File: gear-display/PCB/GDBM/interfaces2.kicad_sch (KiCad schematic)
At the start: 1 part

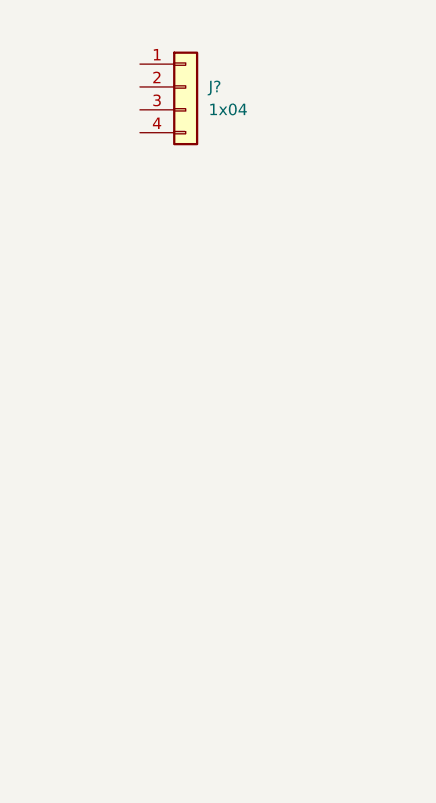
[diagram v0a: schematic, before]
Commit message: updates
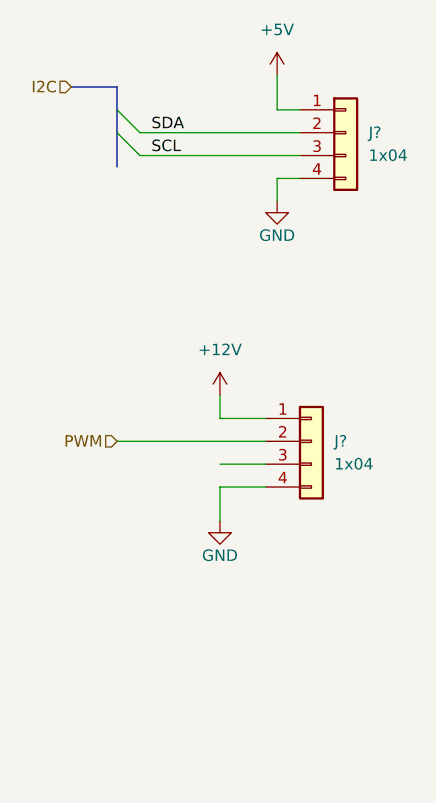
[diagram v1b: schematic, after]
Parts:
- added J?: Con_Screw_1x04_691313510004, KD_Connector_Screw:CON_508_1X04_691313510004_Mated, symbol KD_Connector_Screw:Con_Screw_1x04_691313510004
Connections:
- net +5V: now reaches J?.1 (Pin_1)
- net SDA: now reaches J?.2 (Pin_2)
- net SCL: now reaches J?.3 (Pin_3)
- net GND: now reaches J?.4 (Pin_4)
- net GND: now also J?.4 (Pin_4)
- new net +12V: J?.1 (Pin_1)
- new net PWM: J?.2 (Pin_2)
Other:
- moved on the sheet: J?
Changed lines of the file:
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@@
 (kicad_sch (version 20211123) (generator eeschema)
   (paper "A4")
-  (symbol (lib_id "KD_Connector_Screw:Con_Screw_1x04_691313510004") (at 166.37 53.34 0) (unit 1)
+  (bus_entry (at 163.83 58.42) (size 2.54 2.54)
+    (stroke (width 0) (type default) (color 0 0 0 0))
+  )
+  (bus_entry (at 163.83 60.96) (size 2.54 2.54)
+    (stroke (width 0) (type default) (color 0 0 0 0))
+  )
+  (wire (pts (xy 184.15 58.42) (xy 181.61 58.42))
+    (stroke (width 0) (type default) (color 0 0 0 0))
+  )
+  (bus (pts (xy 163.83 58.42) (xy 163.83 60.96))
+    (stroke (width 0) (type default) (color 0 0 0 0))
+  )
+  (wire (pts (xy 181.61 54.61) (xy 181.61 58.42))
+    (stroke (width 0) (type default) (color 0 0 0 0))
+  )
+  (wire (pts (xy 175.26 92.71) (xy 180.34 92.71))
+    (stroke (width 0) (type default) (color 0 0 0 0))
+  )
+  (wire (pts (xy 163.83 95.25) (xy 180.34 95.25))
+    (stroke (width 0) (type default) (color 0 0 0 0))
+  )
+  (bus (pts (xy 163.83 60.96) (xy 163.83 64.77))
+    (stroke (width 0) (type default) (color 0 0 0 0))
+  )
+  (wire (pts (xy 166.37 63.5) (xy 184.15 63.5))
+    (stroke (width 0) (type default) (color 0 0 0 0))
+  )
+  (wire (pts (xy 180.34 100.33) (xy 175.26 100.33))
+    (stroke (width 0) (type default) (color 0 0 0 0))
+  )
+  (wire (pts (xy 166.37 60.96) (xy 184.15 60.96))
+    (stroke (width 0) (type default) (color 0 0 0 0))
+  )
+  (wire (pts (xy 175.26 100.33) (xy 175.26 104.14))
+    (stroke (width 0) (type default) (color 0 0 0 0))
+  )
+  (wire (pts (xy 175.26 90.17) (xy 175.26 92.71))
+    (stroke (width 0) (type default) (color 0 0 0 0))
+  )
+  (wire (pts (xy 175.26 97.79) (xy 180.34 97.79))
+    (stroke (width 0) (type default) (color 0 0 0 0))
+  )
+  (wire (pts (xy 181.61 66.04) (xy 181.61 68.58))
+    (stroke (width 0) (type default) (color 0 0 0 0))
+  )
+  (bus (pts (xy 163.83 55.88) (xy 163.83 58.42))
+    (stroke (width 0) (type default) (color 0 0 0 0))
+  )
+  (wire (pts (xy 184.15 66.04) (xy 181.61 66.04))
+    (stroke (width 0) (type default) (color 0 0 0 0))
+  )
+  (bus (pts (xy 158.75 55.88) (xy 163.83 55.88))
+    (stroke (width 0) (type default) (color 0 0 0 0))
+  )
+  (label "SCL" (at 167.64 63.5 0)
+    (effects (font (size 1.27 1.27)) (justify left bottom))
+  )
+  (label "SDA" (at 167.64 60.96 0)
+    (effects (font (size 1.27 1.27)) (justify left bottom))
+  )
+  (hierarchical_label "PWM" (shape input) (at 163.83 95.25 180)
+    (effects (font (size 1.27 1.27)) (justify right))
+  )
+  (hierarchical_label "I2C" (shape input) (at 158.75 55.88 180)
+    (effects (font (size 1.27 1.27)) (justify right))
+  )
+  (symbol (lib_id "power:+12V") (at 175.26 90.17 0) (unit 1)
     (in_bom yes) (on_board yes) (fields_autoplaced)
-    (property "Reference" "J?" (id 0) (at 173.99 55.8799 0)
+    (property "Reference" "#PWR?" (id 0) (at 175.26 93.98 0)
+      (effects (font (size 1.27 1.27)) hide)
+    )
+    (property "Value" "+12V" (id 1) (at 175.26 85.09 0))
+    (property "Footprint" "" (id 2) (at 175.26 90.17 0)
+      (effects (font (size 1.27 1.27)) hide)
+    )
+    (property "Datasheet" "" (id 3) (at 175.26 90.17 0)
+      (effects (font (size 1.27 1.27)) hide)
+    )
+    (pin "1")
+  )
+  (symbol (lib_id "power:GND") (at 175.26 104.14 0) (mirror y) (unit 1)
+    (in_bom yes) (on_board yes)
+    (property "Reference" "#PWR?" (id 0) (at 175.26 110.49 0)
+      (effects (font (size 1.27 1.27)) hide)
+    )
+    (property "Value" "GND" (id 1) (at 175.26 107.95 0))
+    (property "Footprint" "" (id 2) (at 175.26 104.14 0)
+      (effects (font (size 1.27 1.27)) hide)
+    )
+    (property "Datasheet" "" (id 3) (at 175.26 104.14 0)
+      (effects (font (size 1.27 1.27)) hide)
+    )
+    (pin "1")
+  )
+  (symbol (lib_id "power:GND") (at 181.61 68.58 0) (mirror y) (unit 1)
+    (in_bom yes) (on_board yes)
+    (property "Reference" "#PWR?" (id 0) (at 181.61 74.93 0)
+      (effects (font (size 1.27 1.27)) hide)
+    )
+    (property "Value" "GND" (id 1) (at 181.61 72.39 0))
+    (property "Footprint" "" (id 2) (at 181.61 68.58 0)
+      (effects (font (size 1.27 1.27)) hide)
+    )
+    (property "Datasheet" "" (id 3) (at 181.61 68.58 0)
+      (effects (font (size 1.27 1.27)) hide)
+    )
+    (pin "1")
+  )
+  (symbol (lib_id "power:+5V") (at 181.61 54.61 0) (unit 1)
+    (in_bom yes) (on_board yes) (fields_autoplaced)
+    (property "Reference" "#PWR?" (id 0) (at 181.61 58.42 0)
+      (effects (font (size 1.27 1.27)) hide)
+    )
+    (property "Value" "+5V" (id 1) (at 181.61 49.53 0))
+    (property "Footprint" "" (id 2) (at 181.61 54.61 0)
+      (effects (font (size 1.27 1.27)) hide)
+    )
+    (property "Datasheet" "" (id 3) (at 181.61 54.61 0)
+      (effects (font (size 1.27 1.27)) hide)
+    )
+    (pin "1")
+  )
+  (symbol (lib_id "KD_Connector_Screw:Con_Screw_1x04_691313510004") (at 180.34 92.71 0) (unit 1)
+    (in_bom yes) (on_board yes) (fields_autoplaced)
+    (property "Reference" "J?" (id 0) (at 187.96 95.2499 0)
       (effects (font (size 1.27 1.27)) (justify left))
     )
-    (property "Value" "Con_Screw_1x04_691313510004" (id 1) (at 153.67 21.59 0)
+    (property "Value" "Con_Screw_1x04_691313510004" (id 1) (at 167.64 60.96 0)
       (effects (font (size 1.27 1.27)) (justify left) hide)
     )
-    (property "Footprint" "KD_Connector_Screw:CON_508_1X04_691313510004_Mated" (id 2) (at 153.67 39.37 0)
+    (property "Footprint" "KD_Connector_Screw:CON_508_1X04_691313510004_Mated" (id 2) (at 167.64 78.74 0)
       (effects (font (size 1.27 1.27)) (justify left) hide)
     )
-    (property "Datasheet" "https://www.we-online.com/katalog/datasheet/6913135100xx.pdf" (id 3) (at 153.67 41.91 0)
+    (property "Datasheet" "https://www.we-online.com/katalog/datasheet/6913135100xx.pdf" (id 3) (at 167.64 81.28 0)
       (effects (font (size 1.27 1.27)) (justify left) hide)
     )
-    (property "Code" "1x04" (id 4) (at 173.99 58.4199 0)
+    (property "Code" "1x04" (id 4) (at 187.96 97.7899 0)
       (effects (font (size 1.27 1.27)) (justify left))
     )
-    (property "Manufacturer" "Würth Elektronik" (id 5) (at 153.67 24.13 0)
+    (property "Manufacturer" "Würth Elektronik" (id 5) (at 167.64 63.5 0)
       (effects (font (size 1.27 1.27)) (justify left) hide)
     )
-    (property "MFG_PartNo" "691313510004" (id 6) (at 153.67 26.67 0)
+    (property "MFG_PartNo" "691313510004" (id 6) (at 167.64 66.04 0)
       (effects (font (size 1.27 1.27)) (justify left) hide)
     )
-    (property "Supplier" "Digi-Key" (id 7) (at 153.67 29.21 0)
+    (property "Supplier" "Digi-Key" (id 7) (at 167.64 68.58 0)
       (effects (font (size 1.27 1.27)) (justify left) hide)
     )
-    (property "Supplier_PartNo" "732-2072-ND" (id 8) (at 153.67 31.75 0)
+    (property "Supplier_PartNo" "732-2072-ND" (id 8) (at 167.64 71.12 0)
       (effects (font (size 1.27 1.27)) (justify left) hide)
     )
-    (property "DNP" "F" (id 9) (at 153.67 34.29 0)
+    (property "DNP" "F" (id 9) (at 167.64 73.66 0)
       (effects (font (size 1.27 1.27)) (justify left) hide)
     )
-    (property "Price" "0.3" (id 10) (at 153.67 36.83 0)
+    (property "Price" "0.3" (id 10) (at 167.64 76.2 0)
       (effects (font (size 1.27 1.27)) (justify left) hide)
     )
+    (pin "1")
+    (pin "2")
+    (pin "3")
+    (pin "4")
+  )
+  (symbol (lib_id "KD_Connector_Screw:Con_Screw_1x04_691313510004") (at 184.15 58.42 0) (unit 1)
+    (in_bom yes) (on_board yes) (fields_autoplaced)
+    (property "Reference" "J?" (id 0) (at 191.77 60.9599 0)
+      (effects (font (size 1.27 1.27)) (justify left))
+    )
+    (property "Value" "Con_Screw_1x04_691313510004" (id 1) (at 171.45 26.67 0)
+      (effects (font (size 1.27 1.27)) (justify left) hide)
+    )
+    (property "Footprint" "KD_Connector_Screw:CON_508_1X04_691313510004_Mated" (id 2) (at 171.45 44.45 0)
+      (effects (font (size 1.27 1.27)) (justify left) hide)
+    )
+    (property "Datasheet" "https://www.we-online.com/katalog/datasheet/6913135100xx.pdf" (id 3) (at 171.45 46.99 0)
+      (effects (font (size 1.27 1.27)) (justify left) hide)
+    )
+    (property "Code" "1x04" (id 4) (at 191.77 63.4999 0)
+      (effects (font (size 1.27 1.27)) (justify left))
+    )
+    (property "Manufacturer" "Würth Elektronik" (id 5) (at 171.45 29.21 0)
+      (effects (font (size 1.27 1.27)) (justify left) hide)
+    )
+    (property "MFG_PartNo" "691313510004" (id 6) (at 171.45 31.75 0)
+      (effects (font (size 1.27 1.27)) (justify left) hide)
+    )
+    (property "Supplier" "Digi-Key" (id 7) (at 171.45 34.29 0)
+      (effects (font (size 1.27 1.27)) (justify left) hide)
+    )
+    (property "Supplier_PartNo" "732-2072-ND" (id 8) (at 171.45 36.83 0)
+      (effects (font (size 1.27 1.27)) (justify left) hide)
+    )
+    (property "DNP" "F" (id 9) (at 171.45 39.37 0)
+      (effects (font (size 1.27 1.27)) (justify left) hide)
+    )
+    (property "Price" "0.3" (id 10) (at 171.45 41.91 0)
+      (effects (font (size 1.27 1.27)) (justify left) hide)
+    )

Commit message: updates
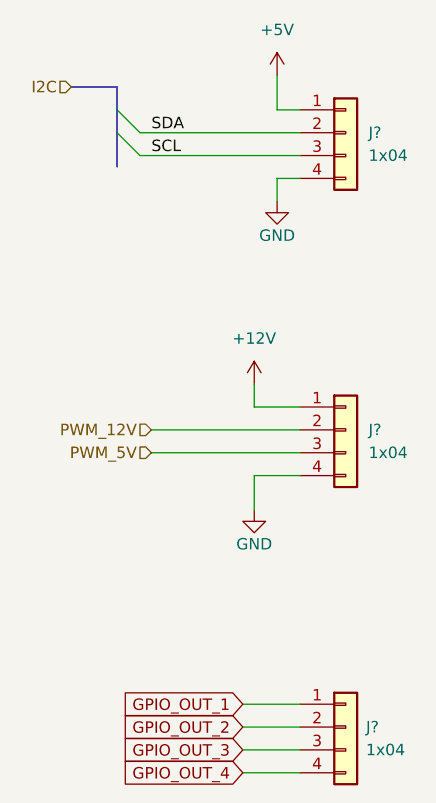
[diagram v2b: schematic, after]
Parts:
- added J?: Con_Screw_1x04_691313510004, KD_Connector_Screw:CON_508_1X04_691313510004_Mated, symbol KD_Connector_Screw:Con_Screw_1x04_691313510004
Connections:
- net PWM_5V: now reaches J?.3 (Pin_3)
- net PWM renamed PWM_12V
- new net GPIO_OUT_1: J?.1 (Pin_1)
- new net GPIO_OUT_2: J?.2 (Pin_2)
- new net GPIO_OUT_3: J?.3 (Pin_3)
- new net GPIO_OUT_4: J?.4 (Pin_4)
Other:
- moved on the sheet: J?
